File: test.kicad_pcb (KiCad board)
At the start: 2 copper layers, 20 x 20 mm, 5 parts, among them U1 STM32F401C_D-E_Ux

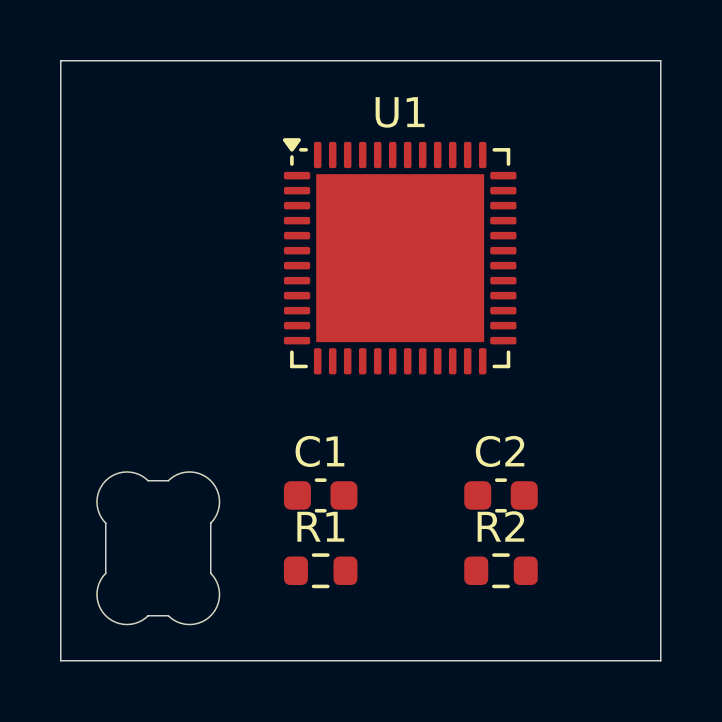
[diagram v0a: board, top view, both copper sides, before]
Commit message: back side
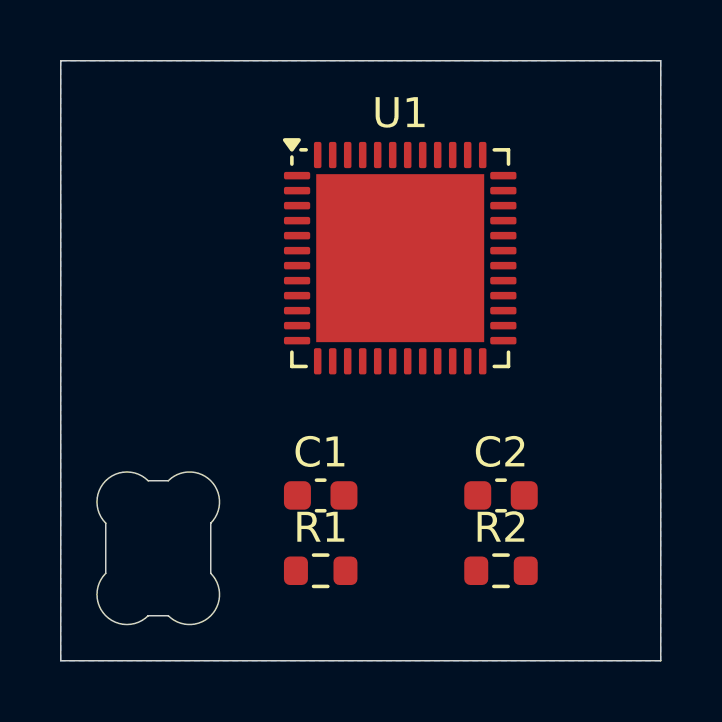
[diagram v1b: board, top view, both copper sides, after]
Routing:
- added copper zone on B.Cu, net (none)
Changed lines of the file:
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@@
 		(layer "Edge.Cuts")
+	)
+	(zone
+		(net 0)
+		(net_name "")
+		(layer "B.Cu")
+		(hatch edge 0.5)
+		(connect_pads
+			(clearance 0.5)
+		)
+		(min_thickness 0.25)
+		(filled_areas_thickness no)
+		(fill yes
+			(mode hatch)
+			(thermal_gap 0.5)
+			(thermal_bridge_width 0.5)
+			(island_removal_mode 1)
+			(island_area_min 10)
+			(hatch_thickness 1)
+			(hatch_gap 1.5)
+			(hatch_orientation 0)
+			(hatch_border_algorithm hatch_thickness)
+			(hatch_min_hole_area 0.3)
+		)
+		(polygon
+			(pts
+				(xy 123 69.5) (xy 123 89.5) (xy 103 89.5) (xy 103 69.5)
+			)
+		)
 	)
 	(embedded_fonts no)
